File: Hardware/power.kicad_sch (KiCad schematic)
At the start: 40 parts, among them IC1 LTC4413EDD#PBF, J3 XT30PW-M, Q1 SISS23DN-T1-GE3, Q6 SSM3K15AMFV,L3F, U3 LM66200DRLR, U4 MAX77827AEFD+T, U5 SC4215ASTRT

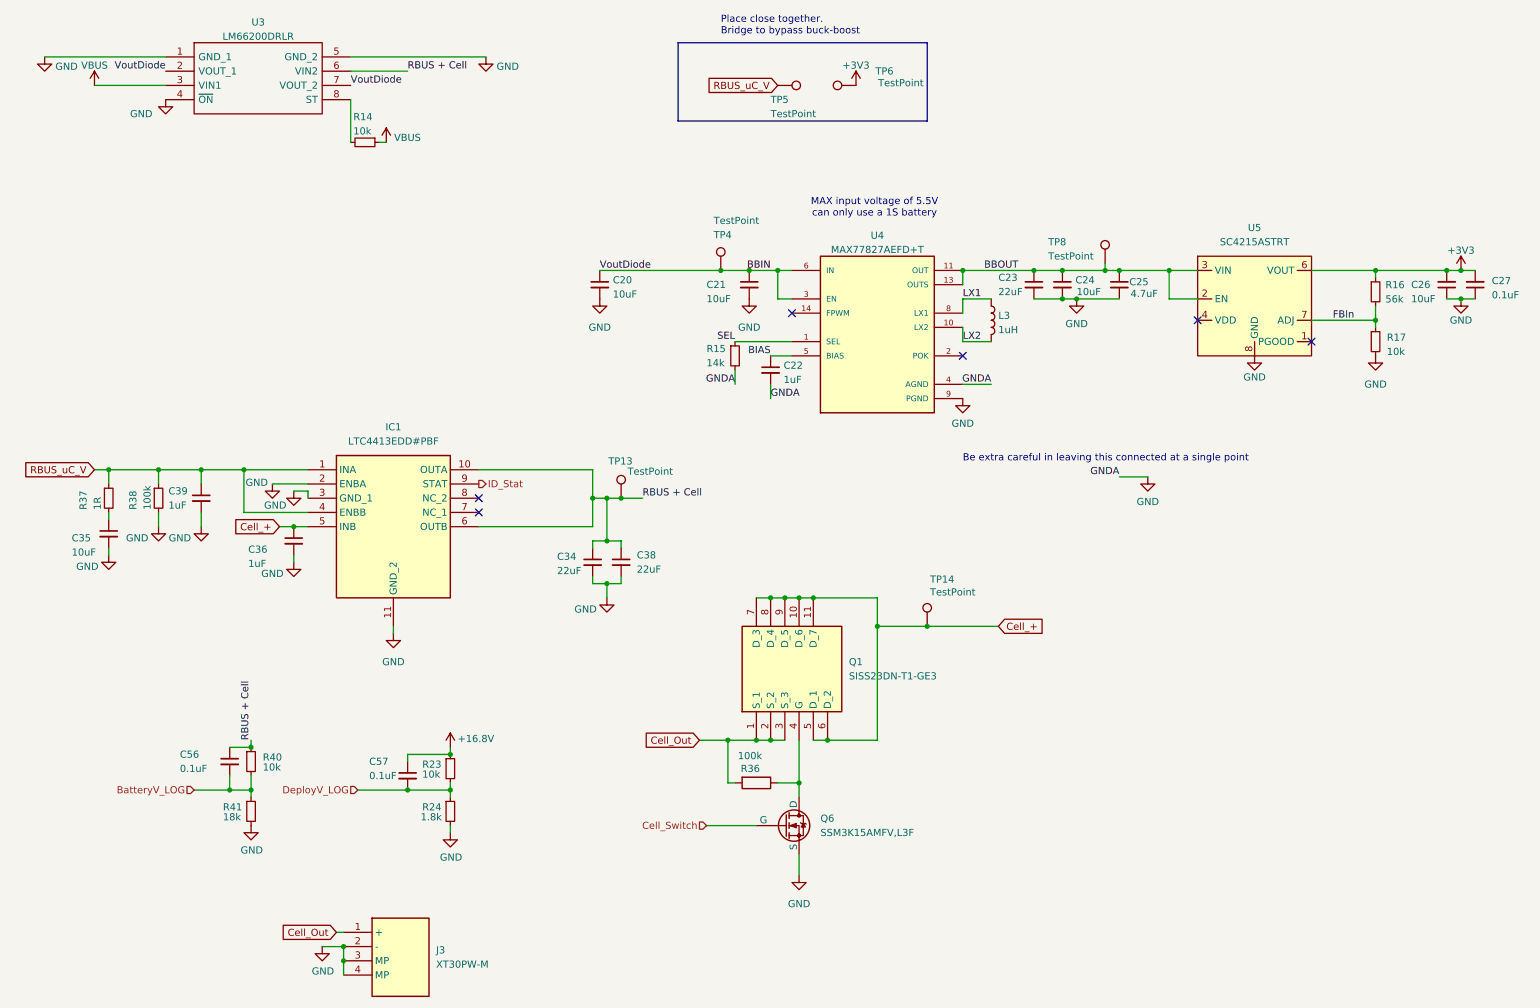
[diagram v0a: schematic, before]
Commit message: Small hardware V2 changes
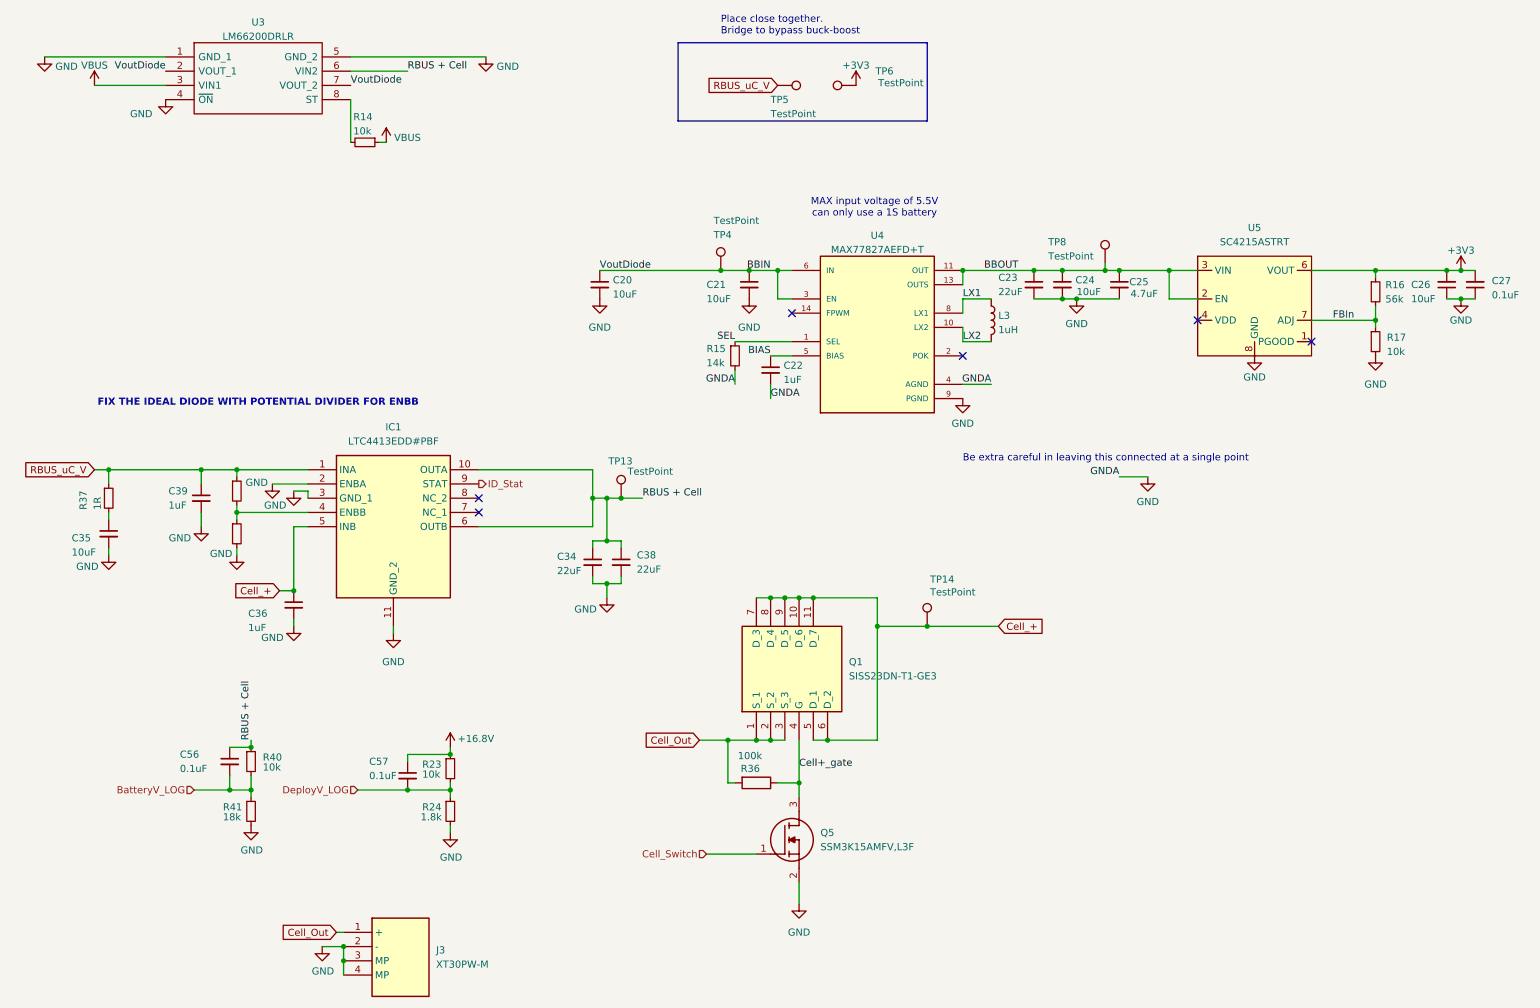
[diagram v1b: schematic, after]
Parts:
- removed Q6: SSM3K15AMFV,L3F, iclr:SOT-723, symbol Simulation_SPICE:NMOS
- removed R38: 100k, Resistor_SMD:R_0402_1005Metric, symbol Device:R_Small
- added Q5: SSM3K15AMFV,L3F, SSM3K15AMFVL3F, symbol iclr:SSM3K15AMFV,L3F
- added R21: R, symbol Device:R_Small
- added R22: R, Resistor_SMD:R_0402_1005Metric, symbol Device:R_Small
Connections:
- net Cell_Switch: now also Q5.1 (G)
- net GND: now also Q5.2 (S), R22.2
- net RBUS_uC_V: now also R21.1; no longer IC1.4 (ENBB)
- net Cell+_gate: now reaches Q1.4 (G), R36.1
- net Cell+_gate: now also Q5.3 (D)
- new net: IC1.4 (ENBB), R21.2, R22.1
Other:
- note added: "FIX THE IDEAL DIODE WITH POTENTIAL DIVIDER FOR ENBB"
- moved on the sheet: C36
